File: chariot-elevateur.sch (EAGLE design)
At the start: 26 parts, among them CON1 XT-60, Q1 BSS138, U1 WIZ820IO

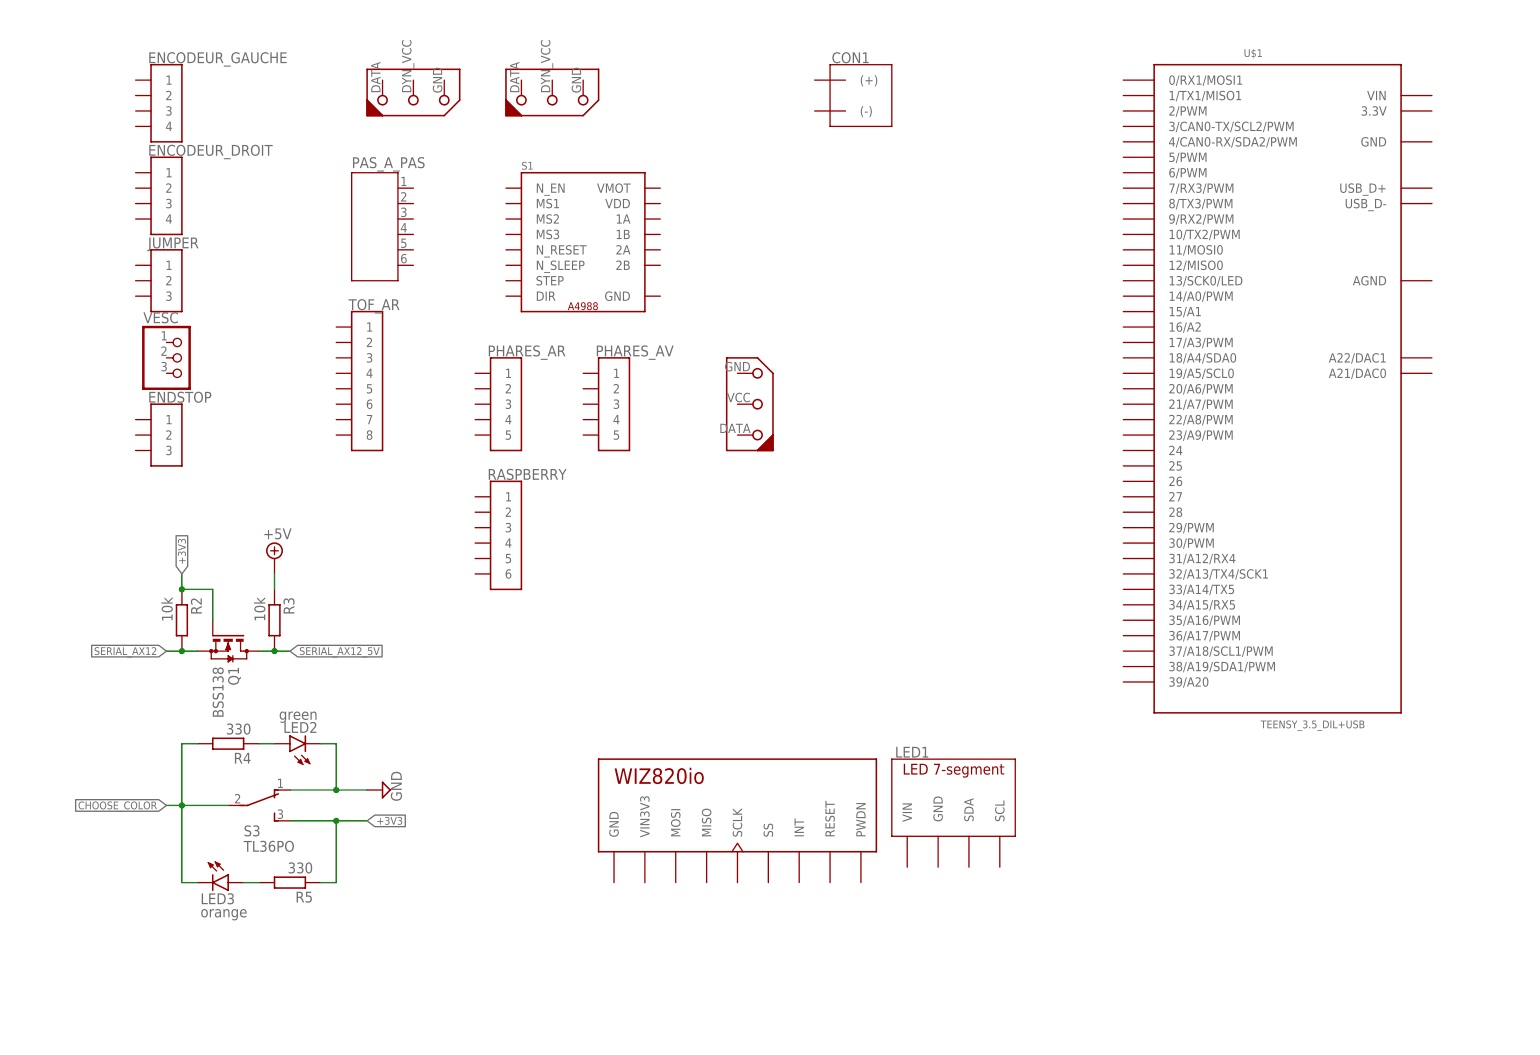
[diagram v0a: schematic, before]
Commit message: end-of-the-day commit
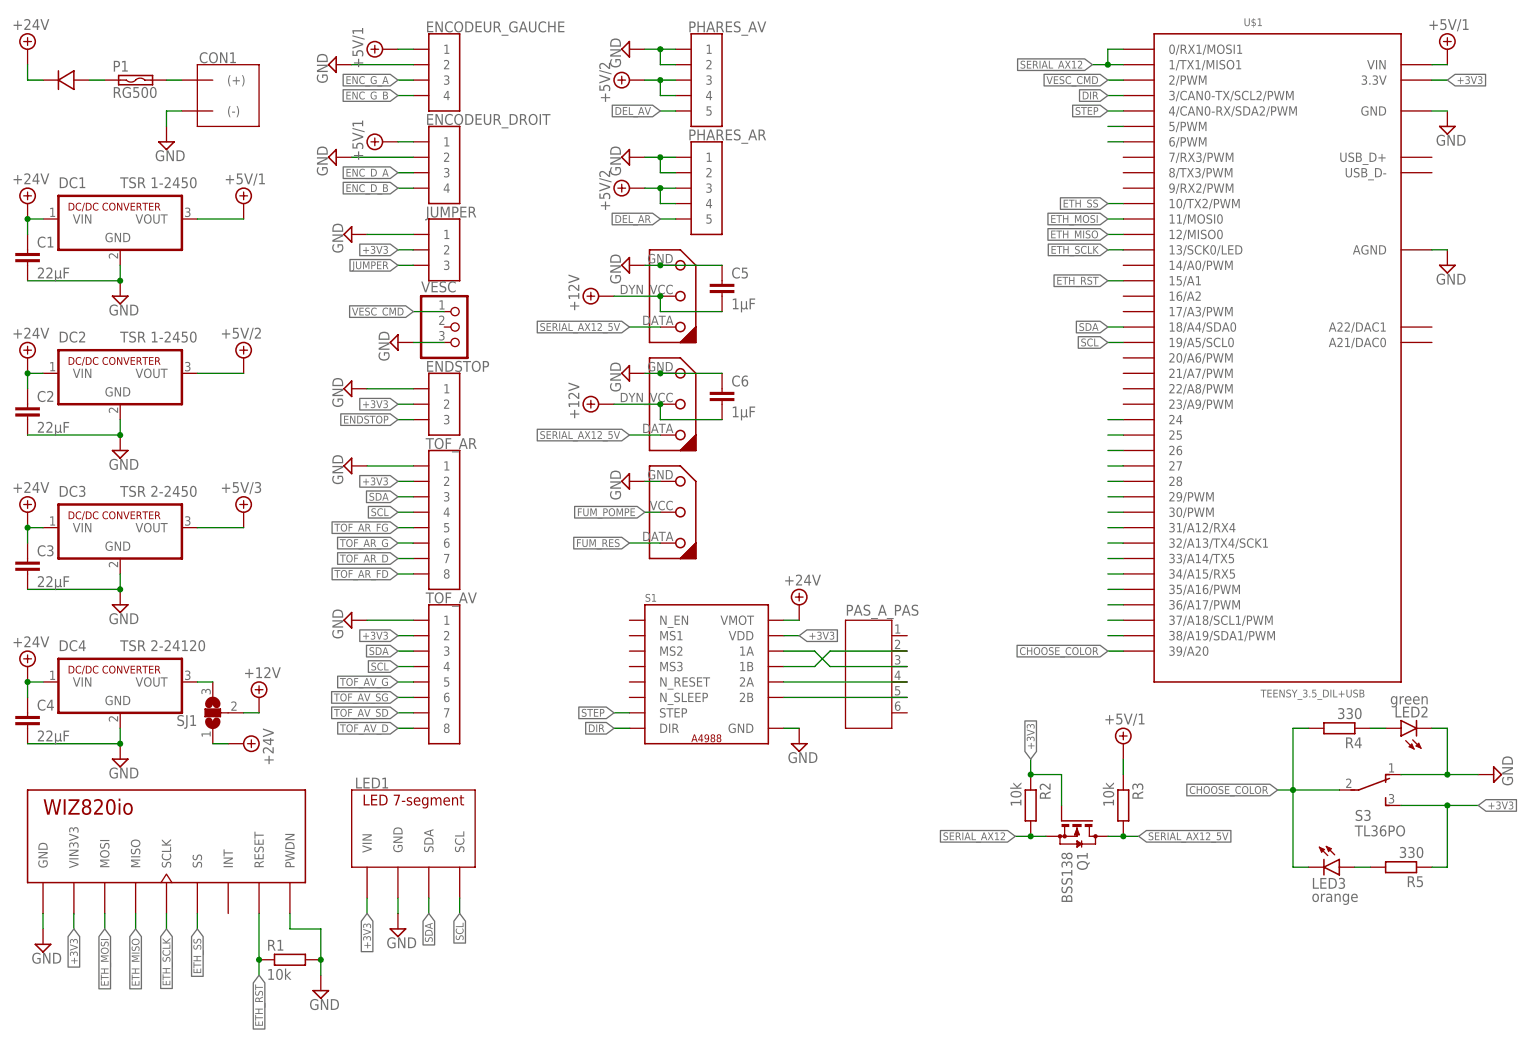
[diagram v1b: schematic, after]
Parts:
- removed RASPBERRY: JST-06, con-jst:JST-06
- added C1, C2, C3, C4: 22µF, resistor:C-EUC0805
- added C5, C6: 1µF, resistor:C-EUC0805
- added D1: DIODE_S15P45, diode_schottky:DIODE_S15P45
- added DC1, DC2: TSR 1-2450, dc-dc-converter:R-78C5.0-1.0
- added DC3: TSR 2-2450, dc-dc-converter:R-78C5.0-1.0
- added DC4: TSR 2-24120, dc-dc-converter:R-78C12-1.0
- added P1: RG500, polyswitch:RGEF800
- added R1: 10k, resistor:R-EU_R0805
- added SJ1: (no value), jumper:SJ2W
- added TOF_AV: JST-08, con-jst:JST-08
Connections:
- removed net +5V: R3.1
- new net +12V: AX12_AR.DYN_VCC, AX12_AV.DYN_VCC, C5.2, C6.2, SJ1.2
- new net +24V: C1.1, C2.1, C3.1, C4.1, D1.-, DC1.VIN, DC2.VIN, DC3.VIN, DC4.VIN, S1.VMOT, SJ1.1
- new net +5V/1: DC1.VOUT, ENCODEUR_DROIT.1, ENCODEUR_GAUCHE.1, R3.1, U$1.VIN
- new net +5V/2: DC2.VOUT, PHARES_AR.3, PHARES_AR.4, PHARES_AV.3, PHARES_AV.4
- new net +5V/3: DC3.VOUT
- new net DEL_AR: PHARES_AR.5
- new net DEL_AV: PHARES_AV.5
- new net DIR: S1.DIR, U$1.3/CAN0-TX/SCL2/PWM
- new net ENC_D_A: ENCODEUR_DROIT.3
- new net ENC_D_B: ENCODEUR_DROIT.4
- new net ENC_G_A: ENCODEUR_GAUCHE.3
- new net ENC_G_B: ENCODEUR_GAUCHE.4
- new net ENDSTOP: ENDSTOP.3
- new net ETH_MISO: U$1.12/MISO0, U1.MISO
- new net ETH_MOSI: U$1.11/MOSI0, U1.MOSI
- new net ETH_RST: R1.1, U$1.15/A1, U1.RESET
- new net ETH_SCLK: U$1.13/SCK0/LED, U1.SCLK
- new net ETH_SS: U$1.10/TX2/PWM, U1.SS
- new net FUM_POMPE: FUMIGENE.DYN_VCC
- new net FUM_RES: FUMIGENE.DATA
- new net JUMPER: JUMPER.3
- new net N$1: CON1.(+), P1.2
- new net N$10: U$1.25
- new net N$11: U$1.26
- new net N$12: U$1.27
- new net N$13: U$1.28
- new net N$14: U$1.29/PWM
- new net N$15: U$1.30/PWM
- new net N$16: U$1.31/A12/RX4
- new net N$17: U$1.32/A13/TX4/SCK1
- new net N$18: U$1.33/A14/TX5
- new net N$19: U$1.34/A15/RX5
- new net N$2: PAS_A_PAS.2, S1.1B
- new net N$20: U$1.35/A16/PWM
- new net N$21: U$1.36/A17/PWM
- new net N$22: U$1.5/PWM
- new net N$23: U$1.6/PWM
- new net N$24: U$1.24
- new net N$25: U$1.37/A18/SCL1/PWM
- new net N$26: U$1.38/A19/SDA1/PWM
- new net N$3: PAS_A_PAS.3, S1.1A
- new net N$4: D1.+, P1.1
- new net N$5: PAS_A_PAS.4, S1.2A
- new net N$6: PAS_A_PAS.5, S1.2B
- new net N$9: DC4.VOUT, SJ1.3
- new net SCL: LED1.SCL, TOF_AR.4, TOF_AV.4, U$1.19/A5/SCL0
- new net SDA: LED1.SDA, TOF_AR.3, TOF_AV.3, U$1.18/A4/SDA0
- new net STEP: S1.STEP, U$1.4/CAN0-RX/SDA2/PWM
- new net TOF_AR_D: TOF_AR.7
- new net TOF_AR_FD: TOF_AR.8
- new net TOF_AR_FG: TOF_AR.5
- new net TOF_AR_G: TOF_AR.6
- new net TOF_AV_D: TOF_AV.8
- new net TOF_AV_G: TOF_AV.5
- new net TOF_AV_SD: TOF_AV.7
- new net TOF_AV_SG: TOF_AV.6
- new net VESC_CMD: U$1.2/PWM, VESC.1
- net +3V3: now also ENDSTOP.2, JUMPER.2, LED1.VIN, S1.VDD, TOF_AR.2, TOF_AV.2, U$1.3.3V, U1.VIN3V3
- net CHOOSE_COLOR: now also U$1.39/A20
- net GND: now also AX12_AR.GND, AX12_AV.GND, C1.2, C2.2, C3.2, C4.2, C5.1, C6.1, CON1.(-), DC1.GND, DC2.GND, DC3.GND, DC4.GND, ENCODEUR_DROIT.2, ENCODEUR_GAUCHE.2, ENDSTOP.1, FUMIGENE.GND, JUMPER.1, LED1.GND, PHARES_AR.1, PHARES_AR.2, PHARES_AV.1, PHARES_AV.2, R1.2, S1.GND, TOF_AR.1, TOF_AV.1, U$1.AGND, U$1.GND, U1.GND, U1.PWDN, VESC.3
- net SERIAL_AX12: now also U$1.0/RX1/MOSI1, U$1.1/TX1/MISO1
- net SERIAL_AX12_5V: now also AX12_AR.DATA, AX12_AV.DATA
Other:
- moved on the sheet: CON1, ENCODEUR_DROIT, ENCODEUR_GAUCHE, ENDSTOP, JUMPER, LED1, LED2, LED3, PAS_A_PAS, PHARES_AR, PHARES_AV, Q1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
